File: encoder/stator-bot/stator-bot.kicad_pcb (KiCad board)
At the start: 4 copper layers, 75.5 x 36.5 mm, 9 parts, among them U1 STM32G474RBTx, U3 TYPE-C_16PIN_2MD(073), U4 XL-1608SURC-06, U5 AZ1117-3.3

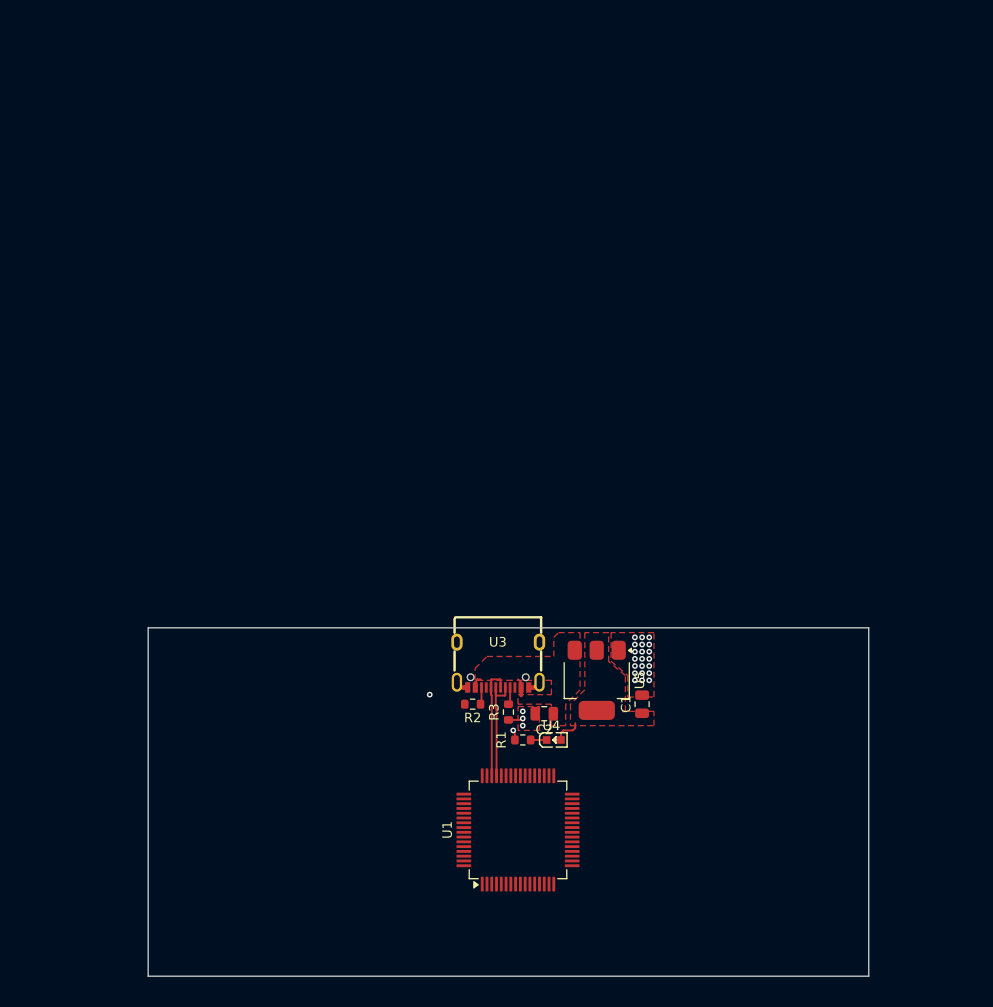
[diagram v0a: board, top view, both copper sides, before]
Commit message: xxx
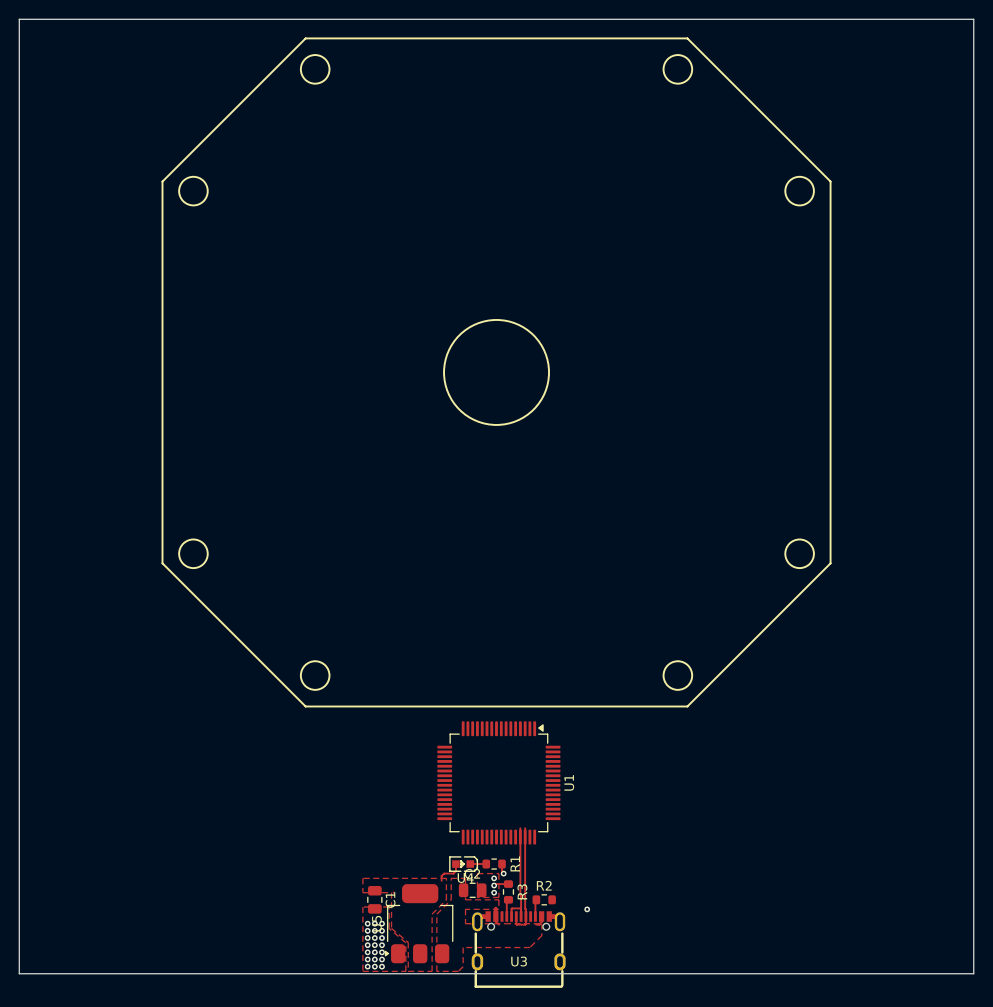
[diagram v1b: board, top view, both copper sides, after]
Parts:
- moved C1 34.7 mm to (75.2, 87.5), turned to -90 degrees
- moved U5 31.5 mm to (80.0, 90.0), turned to 90 degrees
- moved U3 28.8 mm to (90.3, 91.6), turned to 0 degrees
- moved R2 21.8 mm to (93.0, 87.5), turned to 0 degrees
- moved C2 20.0 mm to (85.5, 86.5), turned to 0 degrees
- moved R3 18.8 mm to (89.2, 86.7), turned to 90 degrees
- moved U4 16.1 mm to (84.5, 83.8), turned to 180 degrees
- moved R1 13.3 mm to (87.8, 83.8), turned to 0 degrees
- moved U1 5.32 mm to (88.2, 75.2), turned to -90 degrees
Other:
- board size 75.5 x 36.5 mm -> 100 x 100 mm
